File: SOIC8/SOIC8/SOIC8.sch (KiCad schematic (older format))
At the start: 3 parts, among them J1 Conn_01x04, J2 Conn_01x04, U1 ATtiny85-20SU

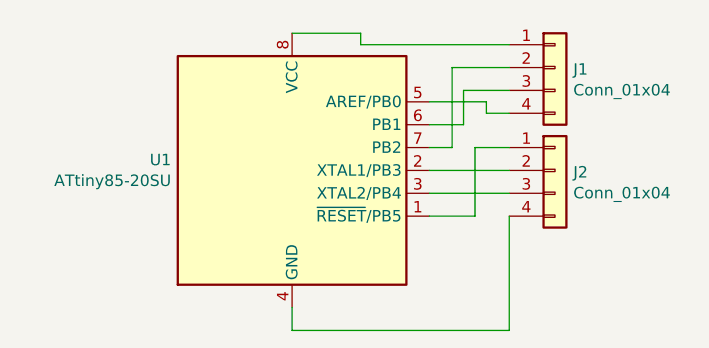
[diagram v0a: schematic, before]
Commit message: Board Updates
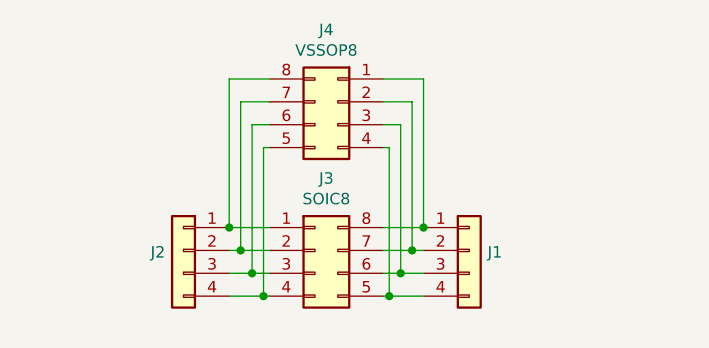
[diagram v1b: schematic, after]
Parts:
- removed U1: ATtiny85-20SU, Package_SO:SOIJ-8_5.3x5.3mm_P1.27mm, symbol MCU_Microchip_ATtiny:ATtiny85-20SU
- added J3: SOIC8, Package_SO:SOIC-8_3.9x4.9mm_P1.27mm, symbol Connector_Generic:Conn_02x04_Counter_Clockwise
- added J4: VSSOP8, Package_SO:VSSOP-8_2.3x2mm_P0.5mm, symbol Connector_Generic:Conn_02x04_Counter_Clockwise
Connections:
- net at J2.1 (Pin_1): now also J3.1 (Pin_1), J4.8 (Pin_8)
- net at J2.2 (Pin_2): now also J3.2 (Pin_2), J4.7 (Pin_7)
- net at J2.3 (Pin_3): now also J3.3 (Pin_3), J4.6 (Pin_6)
- net at J2.4 (Pin_4): now also J3.4 (Pin_4), J4.5 (Pin_5)
- net at J1.4 (Pin_4): now also J3.5 (Pin_5), J4.4 (Pin_4)
- net at J1.3 (Pin_3): now also J3.6 (Pin_6), J4.3 (Pin_3)
- net at J1.2 (Pin_2): now also J3.7 (Pin_7), J4.2 (Pin_2)
- net at J1.1 (Pin_1): now also J3.8 (Pin_8), J4.1 (Pin_1)
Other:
- moved on the sheet: J1, J2
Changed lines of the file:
@@
 Sheet 1 1
 Title "SOIC8 To DIP8 Breakout Board"
-Date "2019-07-04"
-Rev "1"
+Date "2020-02-13"
+Rev "2"
 Comp "SirBoard"
 Comment1 "SOIC8 P = 1.27mm"
-Comment2 "MSOP8 P = 0.65mm"
+Comment2 "VSSOP8 P = 0.5mm"
 Comment3 "DIP8 P = 2.54mm"
 Comment4 ""
 $EndDescr
 $Comp
-L MCU_Microchip_ATtiny:ATtiny85-20SU U1
-U 1 1 5D1B7CEE
-P 2300 1350
-F 0 "U1" H 1771 1396 50  0000 R CNN
-F 1 "ATtiny85-20SU" H 1771 1305 50  0000 R CNN
-F 2 "Package_SO:SOIJ-8_5.3x5.3mm_P1.27mm" H 2300 1350 50  0001 C CIN
-F 3 "http://ww1.microchip.com/downloads/en/DeviceDoc/atmel-2586-avr-8-bit-microcontroller-attiny25-attiny45-attiny85_datasheet.pdf" H 2300 1350 50  0001 C CNN
-	1    2300 1350
-	1    0    0    -1
-$EndComp
-$Comp
 L Connector_Generic:Conn_01x04 J2
 U 1 1 5D1B8092
-P 3450 1350
-F 0 "J2" H 3530 1342 50  0000 L CNN
-F 1 "Conn_01x04" H 3530 1251 50  0000 L CNN
-F 2 "Connector_PinHeader_2.54mm:PinHeader_1x04_P2.54mm_Vertical" H 3450 1350 50  0001 C CNN
-F 3 "~" H 3450 1350 50  0001 C CNN
-	1    3450 1350
-	1    0    0    -1
+P 1825 1700
+F 0 "J2" H 1905 1692 50  0000 L CNN
+F 1 "Conn_01x04" H 1905 1601 50  0001 L CNN
+F 2 "Connector_PinHeader_2.54mm:PinHeader_1x04_P2.54mm_Vertical" H 1825 1700 50  0001 C CNN
+F 3 "~" H 1825 1700 50  0001 C CNN
+	1    1825 1700
+	-1   0    0    -1
 $EndComp
 $Comp
 L Connector_Generic:Conn_01x04 J1
 U 1 1 5D1B8353
-P 3450 900
-F 0 "J1" H 3530 892 50  0000 L CNN
-F 1 "Conn_01x04" H 3530 801 50  0000 L CNN
-F 2 "Connector_PinHeader_2.54mm:PinHeader_1x04_P2.54mm_Vertical" H 3450 900 50  0001 C CNN
-F 3 "~" H 3450 900 50  0001 C CNN
-	1    3450 900
+P 3075 1700
+F 0 "J1" H 3155 1692 50  0000 L CNN
+F 1 "Conn_01x04" H 3155 1601 50  0001 L CNN
+F 2 "Connector_PinHeader_2.54mm:PinHeader_1x04_P2.54mm_Vertical" H 3075 1700 50  0001 C CNN
+F 3 "~" H 3075 1700 50  0001 C CNN
+	1    3075 1700
+	1    0    0    -1
+$EndComp
+$Comp
+L Connector_Generic:Conn_02x04_Counter_Clockwise J4
+U 1 1 5E452362
+P 2500 1050
+F 0 "J4" H 2550 1365 50  0000 C CNN
+F 1 "VSSOP8" H 2550 1275 50  0000 C CNN
+F 2 "Package_SO:VSSOP-8_2.3x2mm_P0.5mm" H 2500 1050 50  0001 C CNN
+F 3 "~" H 2500 1050 50  0001 C CNN
+	1    2500 1050
+	-1   0    0    -1
+$EndComp
+$Comp
+L Connector_Generic:Conn_02x04_Counter_Clockwise J3
+U 1 1 5E452B4C
+P 2400 1700
+F 0 "J3" H 2450 2015 50  0000 C CNN
+F 1 "SOIC8" H 2450 1925 50  0000 C CNN
+F 2 "Package_SO:SOIC-8_3.9x4.9mm_P1.27mm" H 2400 1700 50  0001 C CNN
+F 3 "~" H 2400 1700 50  0001 C CNN
+	1    2400 1700
 	1    0    0    -1
 $EndComp
 Wire Wire Line
-	3250 1250 3100 1250
+	2700 950  2875 950
 Wire Wire Line
-	3100 1250 3100 1550
+	2700 1050 2825 1050
 Wire Wire Line
-	3100 1550 2900 1550
+	2700 1150 2775 1150
 Wire Wire Line
-	2900 1350 3250 1350
+	2775 1150 2775 1800
 Wire Wire Line
-	3250 1450 2900 1450
+	2700 1250 2725 1250
 Wire Wire Line
-	3250 1550 3250 2050
+	2725 1250 2725 1900
 Wire Wire Line
-	3250 2050 2300 2050
+	2700 1700 2825 1700
 Wire Wire Line
-	2300 2050 2300 1950
+	2700 1800 2775 1800
 Wire Wire Line
-	3250 800  2600 800
+	2700 1900 2725 1900
+Connection ~ 2725 1900
+Connection ~ 2775 1800
+Connection ~ 2825 1700
 Wire Wire Line
-	2600 800  2600 750
+	2700 1600 2875 1600
 Wire Wire Line
-	2600 750  2300 750
+	2725 1900 2875 1900
 Wire Wire Line
-	3250 900  3000 900
+	2775 1800 2875 1800
 Wire Wire Line
-	3000 900  3000 1250
+	2825 1700 2875 1700
+Connection ~ 2875 1600
 Wire Wire Line
-	3000 1250 2900 1250
+	2825 1050 2825 1700
 Wire Wire Line
-	3250 1000 3050 1000
+	2875 950  2875 1600
 Wire Wire Line
-	3050 1000 3050 1150
+	2025 950  2025 1600
 Wire Wire Line
-	3050 1150 2900 1150
+	2075 1050 2075 1700
 Wire Wire Line
-	3250 1100 3150 1100
+	2175 1250 2175 1900
 Wire Wire Line
-	3150 1100 3150 1050
+	2200 1250 2175 1250
 Wire Wire Line
-	3150 1050 2900 1050
+	2125 1150 2125 1800
+Wire Wire Line
+	2200 1150 2125 1150
+Wire Wire Line
+	2200 1050 2075 1050
+Wire Wire Line
+	2200 950  2025 950
+Wire Wire Line
+	2200 1600 2025 1600
+Connection ~ 2025 1600
+Wire Wire Line
+	2025 1700 2075 1700
+Connection ~ 2075 1700
+Wire Wire Line
+	2075 1700 2200 1700
+Wire Wire Line
+	2200 1800 2125 1800
+Connection ~ 2125 1800
+Wire Wire Line
+	2125 1800 2025 1800
+Wire Wire Line
+	2025 1900 2175 1900
+Connection ~ 2175 1900
+Wire Wire Line
+	2175 1900 2200 1900
 $EndSCHEMATC
